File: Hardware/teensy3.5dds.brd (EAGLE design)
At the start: 160 x 101.3 mm, 98 parts, among them IC1 AD8034, IC10 AD8034, IC11 AD8034, IC12 AD8034, IC2 AD8034, IC4 AD737KRZ-R7, IC8 AD8034, IC9 AD8034, J1 1776275-2, J2 1776275-2, Q1 CSM-7X-DU, X1 1-227161-0

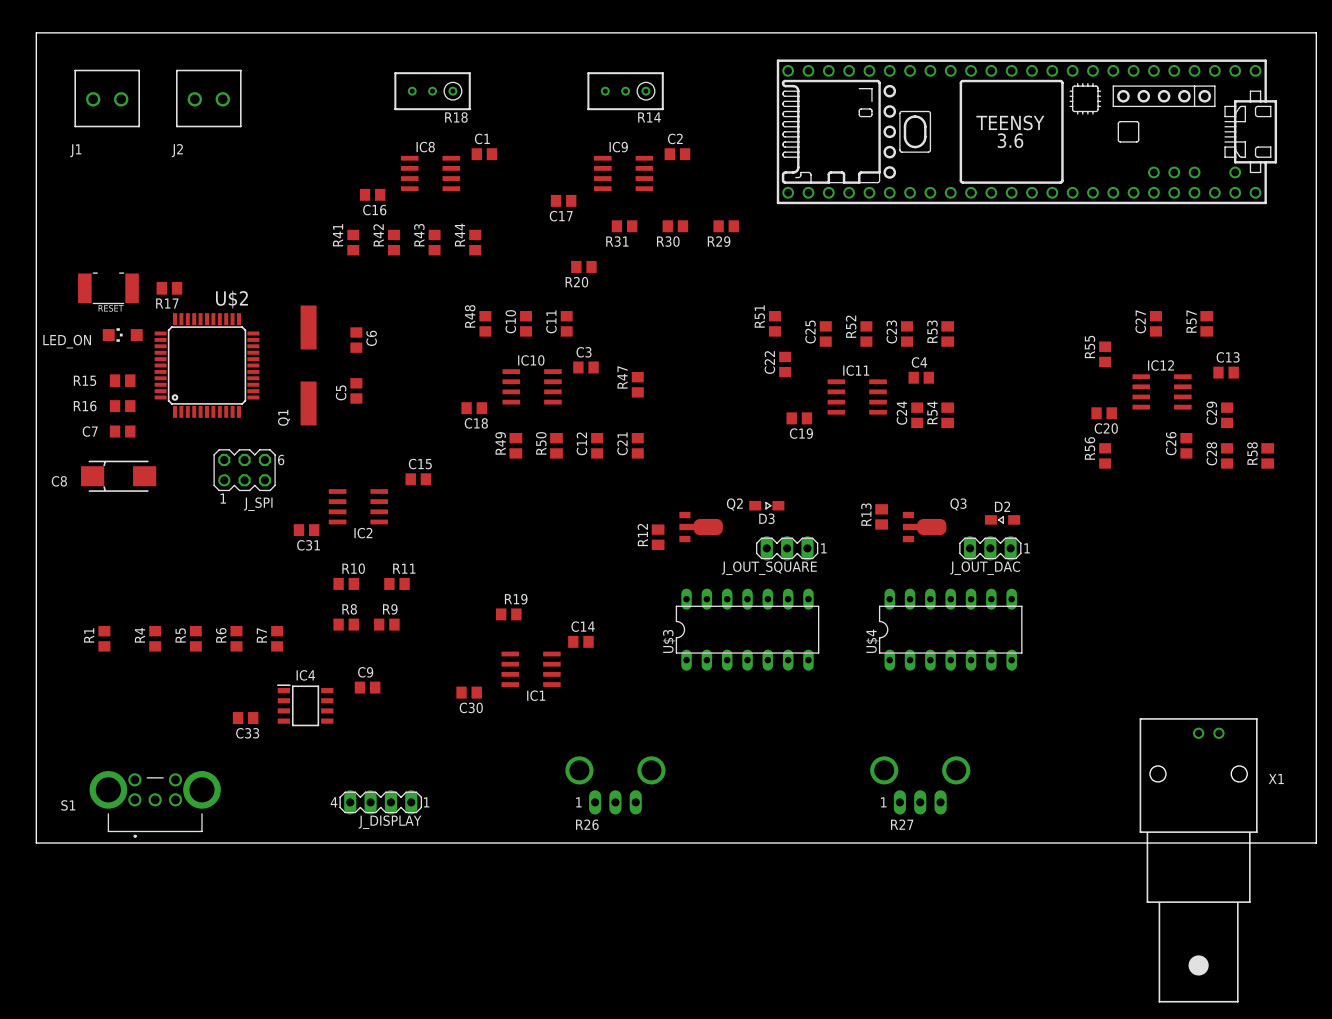
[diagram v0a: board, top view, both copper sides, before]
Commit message: hardware: board v0.1
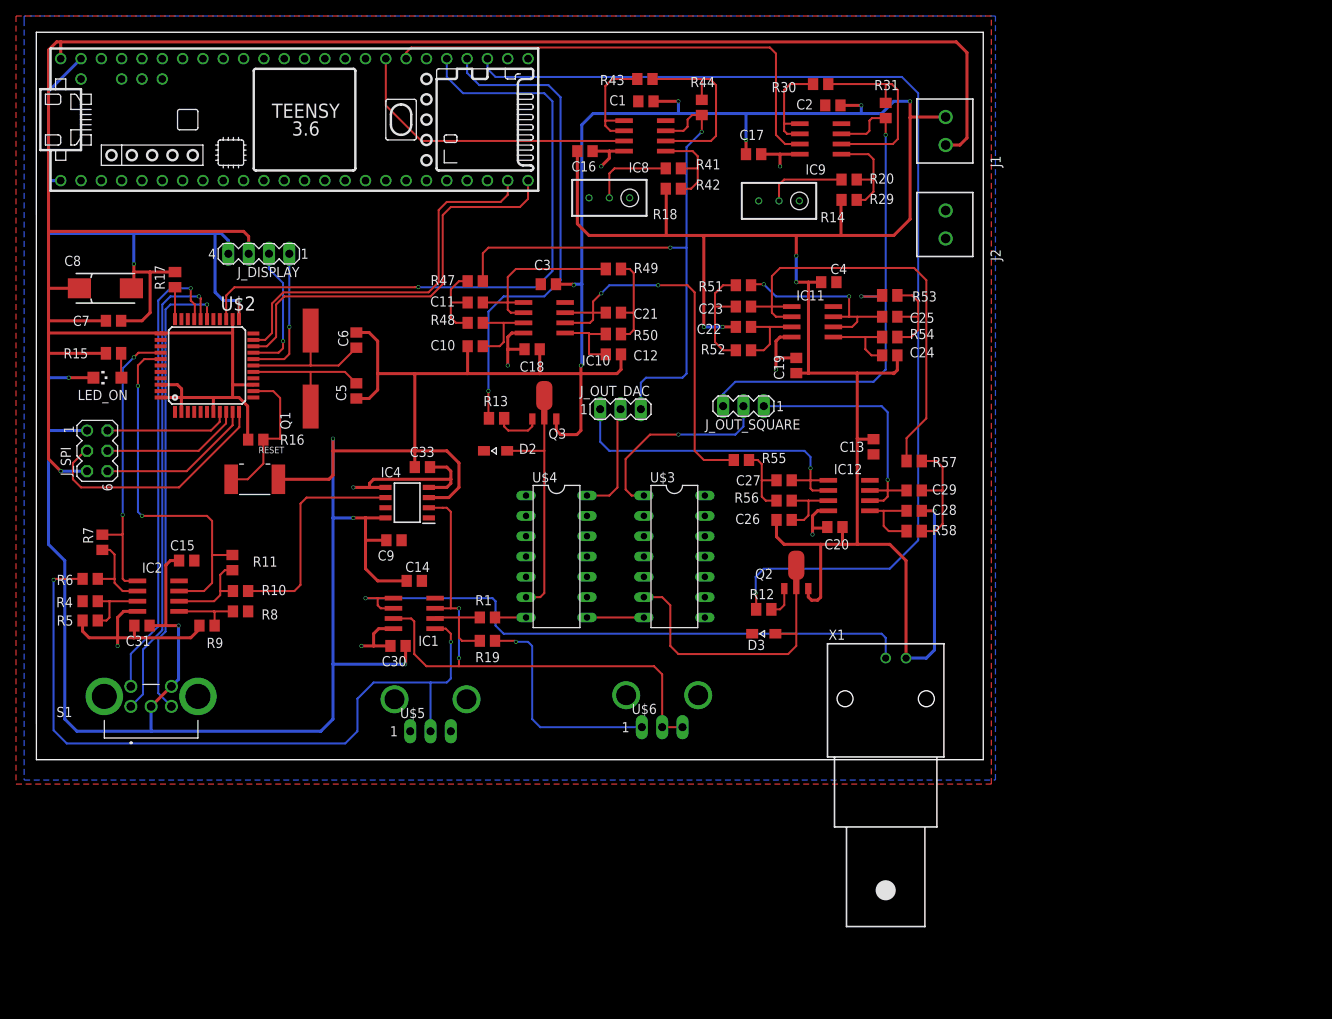
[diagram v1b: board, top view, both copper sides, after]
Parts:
- removed R26, R27: POTENTIOMETER_VERTICAL, Potentiometer_vertical:MA03-1
- added U$5, U$6: POTENTIOMETER_VERTICAL, Potentiometer_vertical:MA03-1
- moved J1 106.7 mm to (113.7, 86.0), turned to 90 degrees
- moved J2 95.5 mm to (113.7, 74.3), turned to 90 degrees
- moved U$1 93.5 mm to (31.0, 89.2), turned to 0 degrees
- moved J_DISPLAY 70.3 mm to (27.8, 72.4)
- moved D2 64.0 mm to (57.4, 47.8)
- moved C26 51.1 mm to (93.5, 39.1), turned to 0 degrees
- moved C27 50.4 mm to (93.5, 44.1), turned to 180 degrees
- moved U$4 50.1 mm to (65.0, 34.5), turned to 270 degrees
- moved Q3 50.0 mm to (63.5, 53.7), turned to 0 degrees
- moved R13 49.7 mm to (57.5, 51.8), turned to 0 degrees
- moved J_OUT_DAC 49.4 mm to (73.0, 53.0), turned to 0 degrees
- moved R1 48.0 mm to (56.4, 26.9), turned to 180 degrees
- moved R55 47.3 mm to (88.1, 46.6), turned to 0 degrees
- moved R58 45.2 mm to (109.7, 37.7), turned to 180 degrees
- moved C13 45.0 mm to (104.6, 48.3), turned to 90 degrees
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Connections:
- removed net N$6: IC1.6, IC1.7, X1.1
- new net N$17: Q2.1, R12.2
- new net N$18: Q3.1, R13.2
- new net N$19: IC1.1, IC1.2, X1.1
- net DAC0_SEL: no longer Q3.1, R13.2
- net GND: no longer U$2.15, U$2.35, U$2.43, U$2.5
- net N$15: now also U$6.1; no longer R26.2
- net N$16: now also IC2.6; no longer IC2.5
- net N$22: now also IC2.5; no longer IC2.6
- net N$3: now also IC1.5, U$5.2; no longer IC1.3, R27.3
- net N$5: now also IC1.6; no longer IC1.2
- net N$67: now also R57.1; no longer R53.1
- net N$70: now also R51.1; no longer R57.1
- net N$9: now also IC1.3, IC1.7, U$6.2, U$6.3; no longer IC1.1, IC1.5, R26.1, R26.3
- net RX1: now also U$1.32/A13; no longer U$1.33/A14
- net SQUARE_OFFSET: now also R53.1; no longer R51.1
- net SQUARE_SEL: no longer Q2.1, R12.2
- net TX1: now also U$1.31/A12; no longer U$1.34/A15
- net V+: now also U$5.3; no longer R27.2
- net V-: now also U$5.1; no longer R27.1
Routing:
- net GND: track 0.00 -> 708.8 mm, vias 0 -> 18
- net +5V: track 0.00 -> 292.4 mm, vias 0 -> 1
- net SQUARE_SEL: track 0.00 -> 138.6 mm, vias 0 -> 1
- net N$3: track 0.00 -> 92.5 mm, vias 0 -> 2
- net V-: track 0.00 -> 90.7 mm, vias 0 -> 8
- net INTERRUPT: track 0.00 -> 83.0 mm, vias 0 -> 1
- net N$19: track 0.00 -> 77.9 mm, vias 0 -> 1
- net DAC0_OFFSET: track 0.00 -> 77.7 mm, vias 0 -> 2
- net N$9: track 0.00 -> 73.3 mm, vias 0 -> 2
- net SQUARE_OFFSET: track 0.00 -> 67.3 mm, vias 0 -> 2
- net DAC0_SEL: track 0.00 -> 61.6 mm, vias 0 -> 1
- net SQUARE: track 0.00 -> 61.2 mm
- net N$8: track 0.00 -> 59.8 mm, vias 0 -> 1
- net N$25: track 0.00 -> 58.4 mm, vias 0 -> 1
- net N$1: track 0.00 -> 57.9 mm, vias 0 -> 1
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- added copper zone on layer 1, net V+
- added copper zone on layer 16, net V-
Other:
- board size 160 x 101.3 mm -> 118.4 x 90.9 mm
